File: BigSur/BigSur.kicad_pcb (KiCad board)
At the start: 2 copper layers, 148 parts, among them J1 XT30PW-M, J10 XT30PW-M, J12 XT30PW-M, J14 XT30PW-M, J15 XT30PW-M, J16 XT30PW-M, J2 XT30PW-M, J3 XT30PW-M, J4 XT30PW-M, J5 XT30PW-M, J6 XT30PW-M, J7 XT30PW-M, J8 XT30PW-M, J9 XT30PW-M, K1 G5LE-1A-VDDC12, K2 G5LE-1A-VDDC12, K3 G5LE-1A-VDDC12, K4 G5LE-1A-VDDC12, Q1 TSM900N10, Q2 TSM900N10, Q3 MMBT3904-7-F, Q4 MMBT3904-7-F, Q5 MMBT3904-7-F, Q6 MMBT3904-7-F, U1 DRV103H, U10 MCP6L02T-E_MS, U11 74LVC1G08W5-7, U12 ACS70331EESATR-2P5U3, U2 DRV103H, U3 DRV8806, U4 SMD46, U5 ACS70331EESATR-2P5U3, U6 ACS70331EESATR-2P5U3, U7 ACS70331EESATR-2P5U3, U8 ACS70331EESATR-2P5U3, U9 ACS70331EESATR-2P5U3

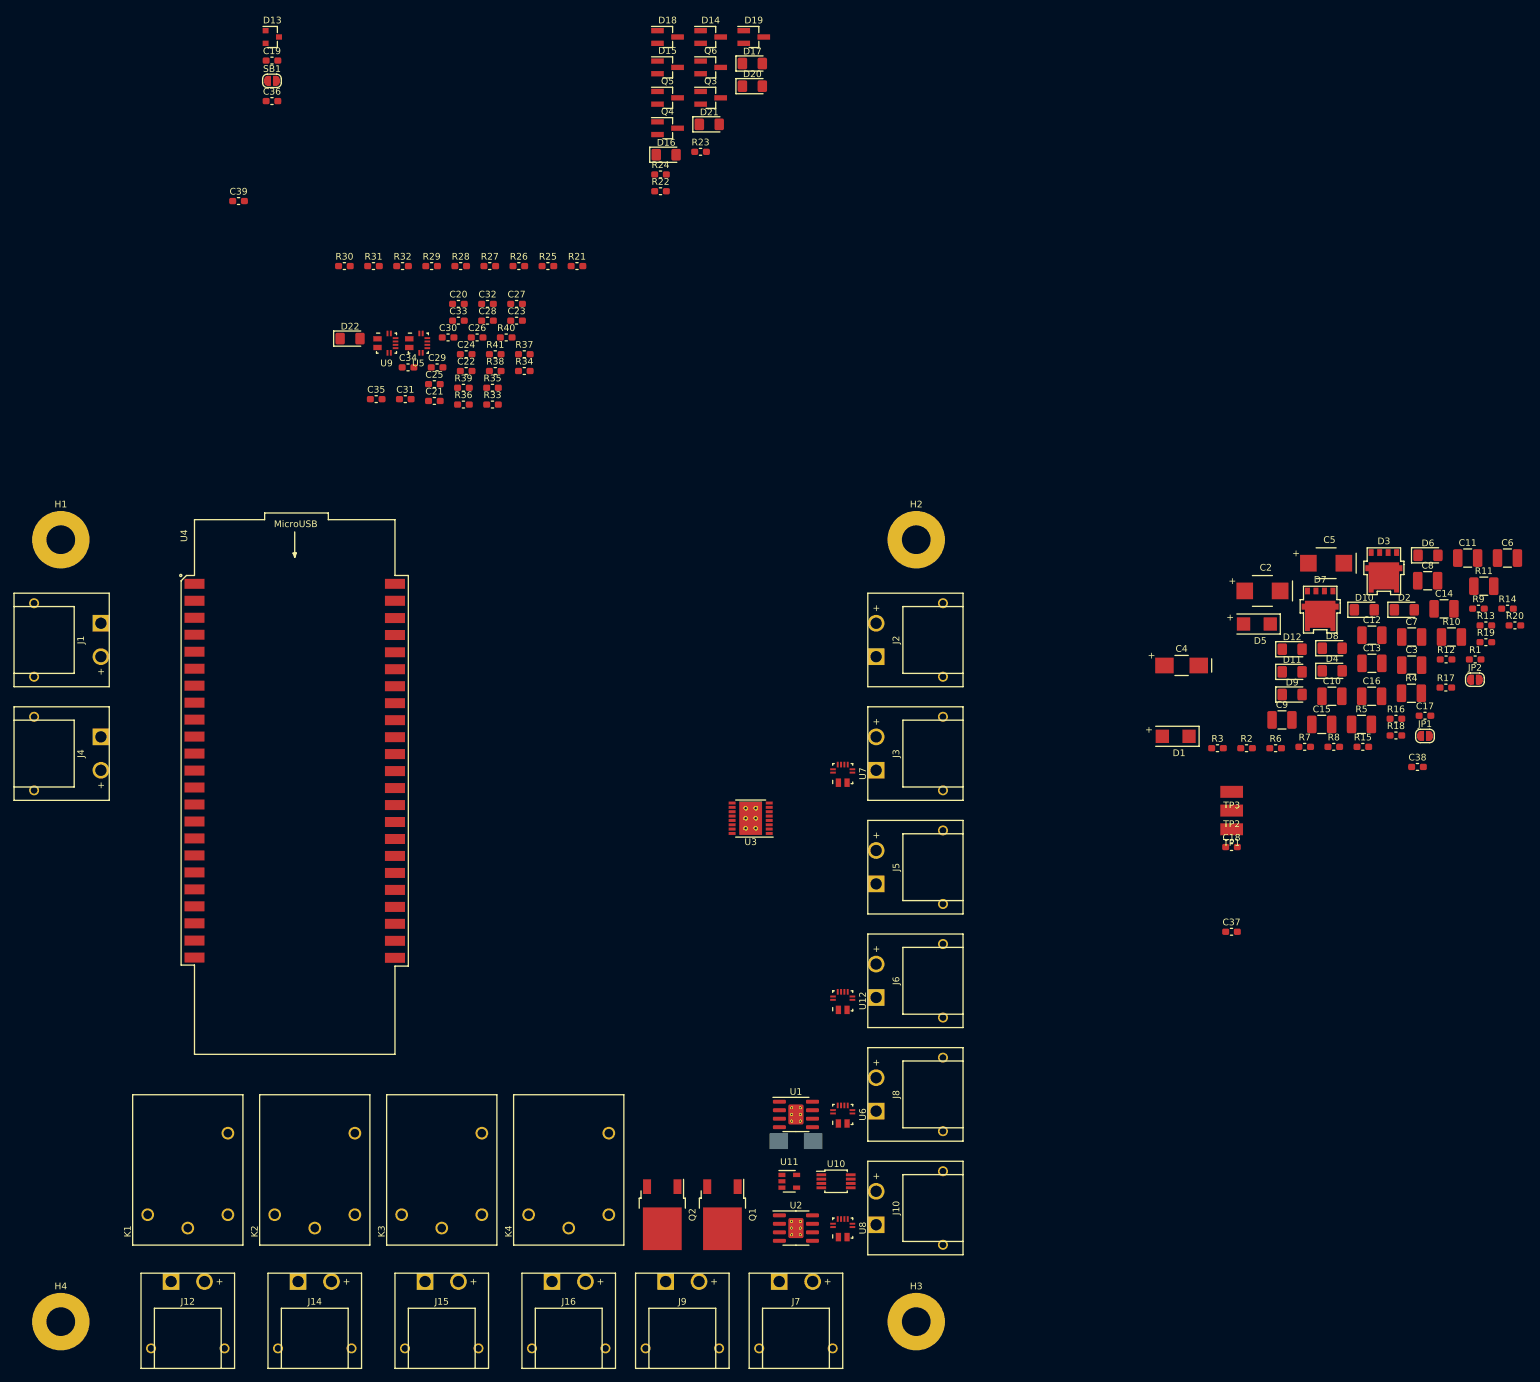
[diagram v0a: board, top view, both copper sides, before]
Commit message: Initial layout pass. This will be changed many times I'm sure.
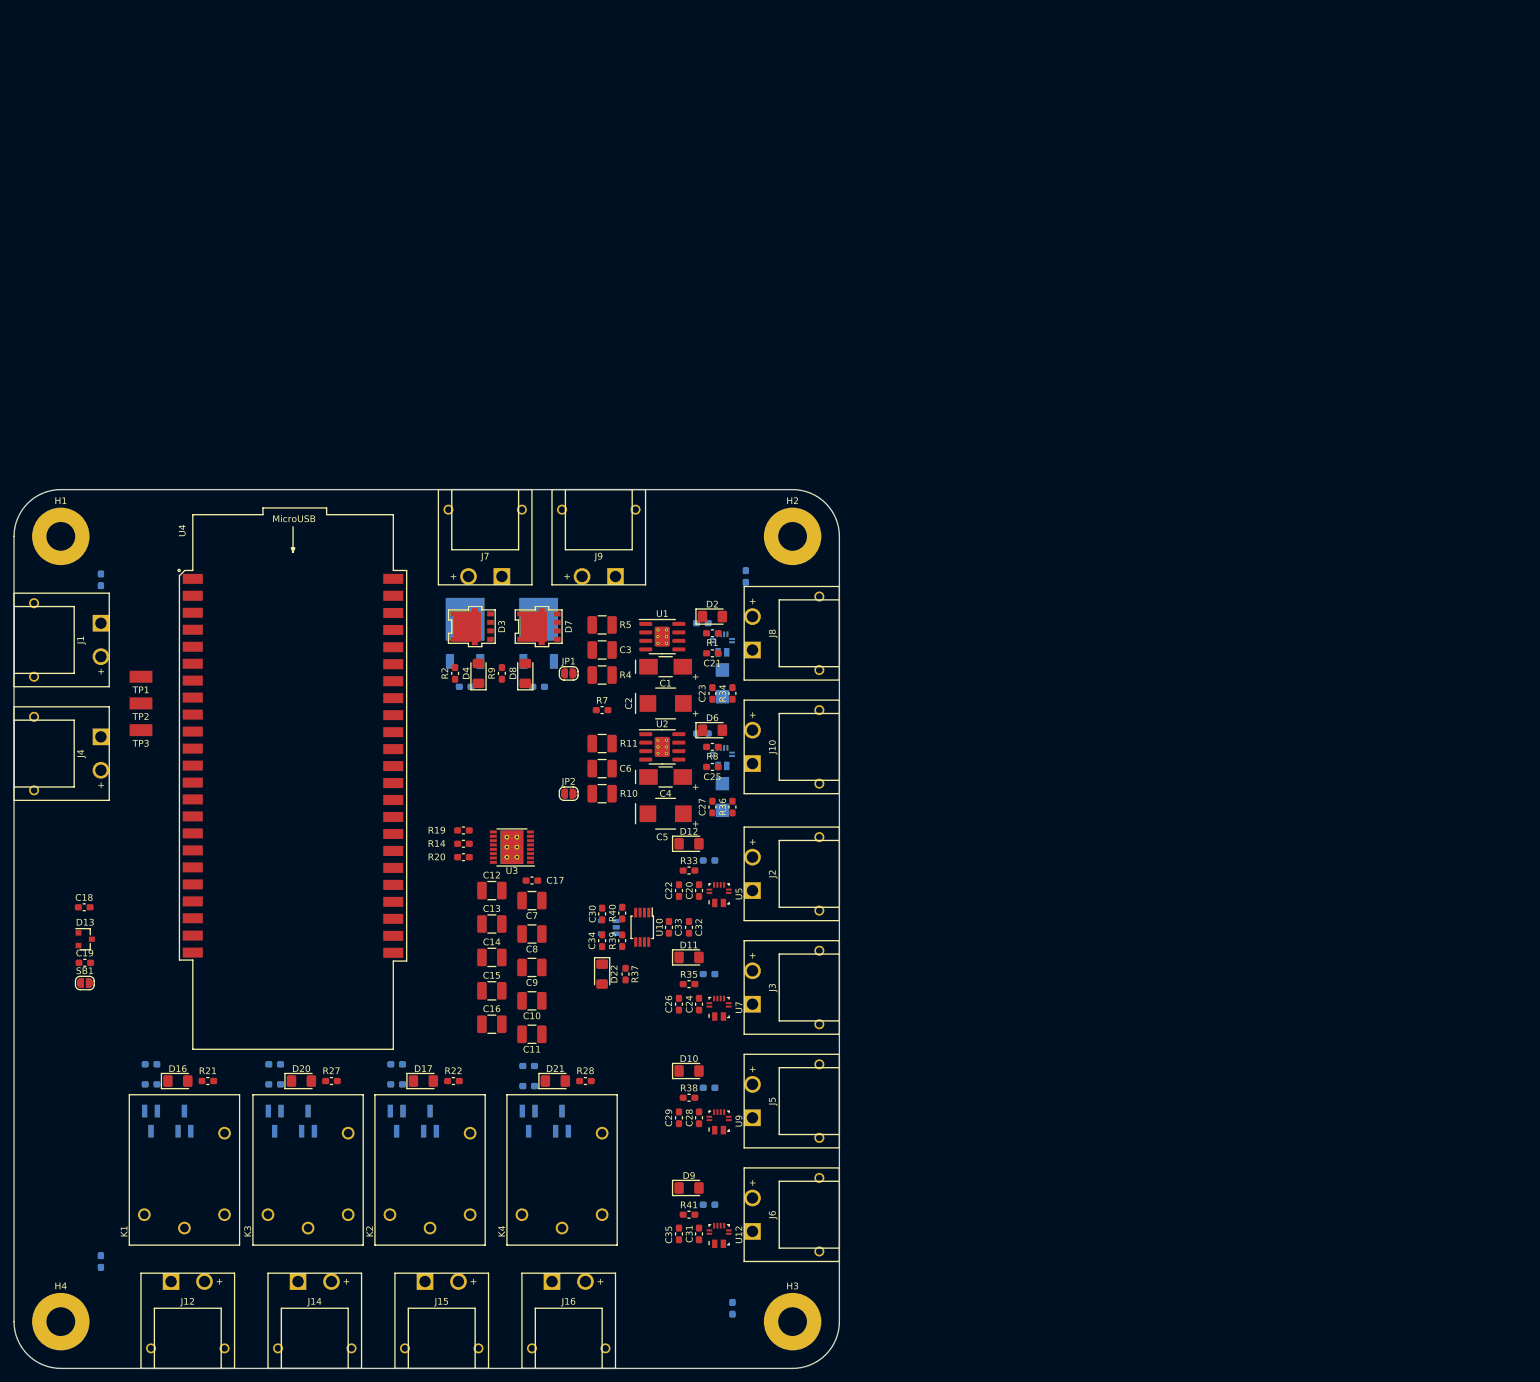
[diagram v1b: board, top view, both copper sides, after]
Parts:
- C1: moved to F.Cu
- C36, C37, C38, C39, D1, D14, D15, D18, D19, D5, Q1, Q2, Q3, Q4, Q5, Q6, R12, R13, R15, R16, R17, R18, R23, R24, R25, R26, R29, R3, R30, R31, R32, R6, U11, U6, U8: moved to B.Cu
- moved D14 180.3 mm to (51.5, 115.0), turned to 90 degrees
- moved Q3 174.5 mm to (46.5, 115.0), turned to 270 degrees
- moved C18 171.9 mm to (36.5, 83.0)
- moved D15 166.6 mm to (70.0, 115.0), turned to 90 degrees
- moved D18 166.1 mm to (88.2, 115.0), turned to 90 degrees
- moved TP1 164.8 mm to (45.0, 48.5)
- moved D19 164.7 mm to (108.0, 115.0), turned to 90 degrees
- moved Q5 164.0 mm to (65.0, 115.0), turned to 270 degrees
- moved TP2 164.0 mm to (45.0, 52.5)
- moved TP3 163.5 mm to (45.0, 56.5)
- moved D20 163.4 mm to (69.0, 109.0)
- moved R20 161.1 mm to (93.2, 75.5)
- moved R14 160.1 mm to (93.2, 73.5), turned to 180 degrees
- moved D17 160.0 mm to (87.2, 109.0)
- moved Q6 160.0 mm to (103.0, 115.0), turned to 270 degrees
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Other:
- board outline added: 123.5 x 131.5 mm
